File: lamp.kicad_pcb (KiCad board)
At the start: 2 copper layers, 83.8 x 40.6 mm, 18 parts, among them J1 Screw_Terminal_01x02, J2 Screw_Terminal_01x02, Q1 2N7002, U1 ESP-12E, U2 34.81-7048, U3 AMS1117-3.3

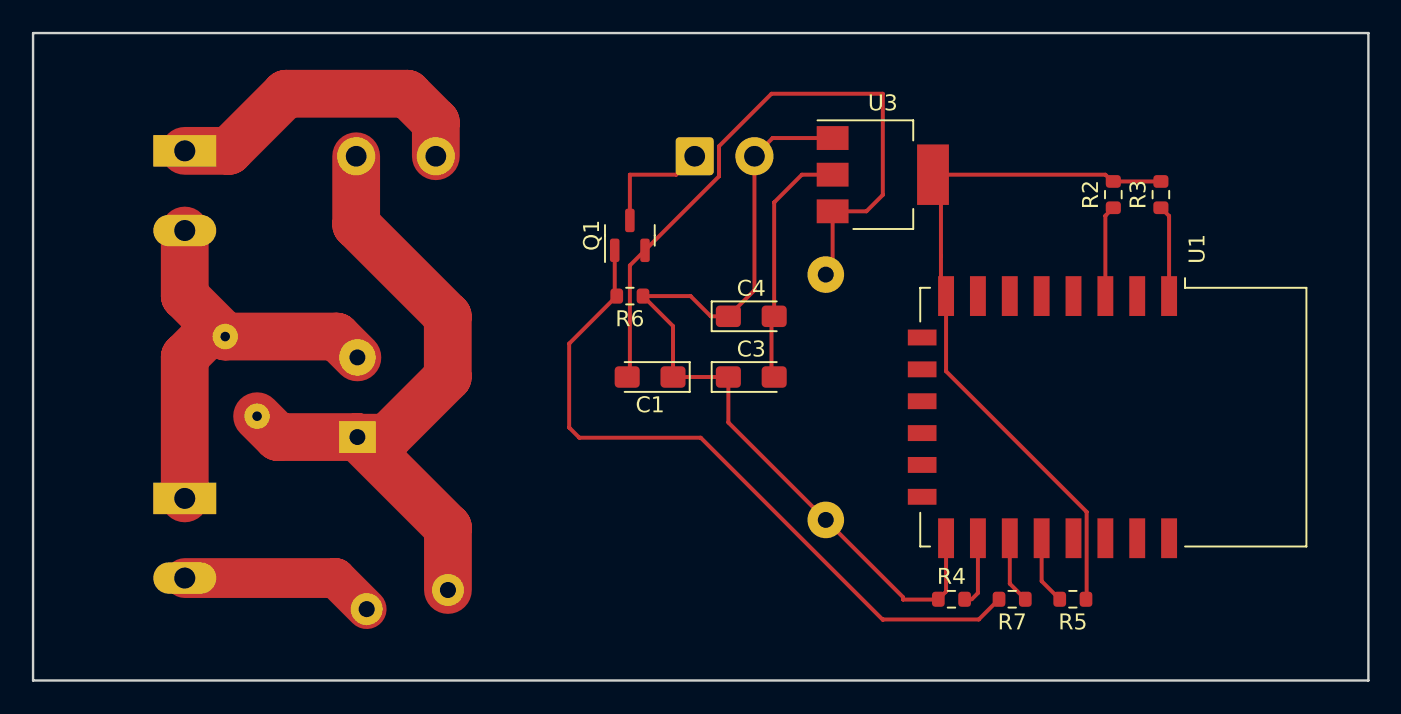
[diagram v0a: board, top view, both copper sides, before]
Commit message: some chnges
some changes
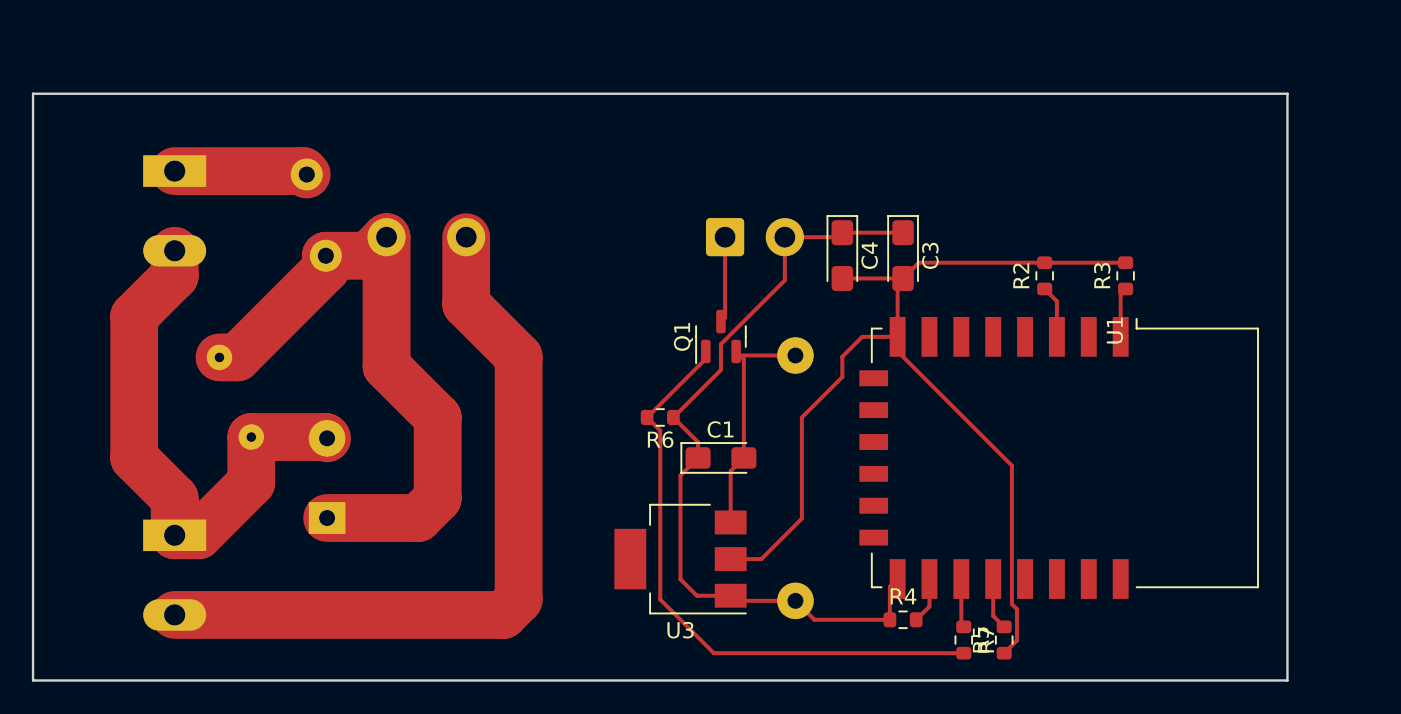
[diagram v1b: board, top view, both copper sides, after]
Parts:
- moved F1 27.5 mm to (130.2, 100.3), turned to -90 degrees
- moved U3 27.3 mm to (153.7, 124.5), turned to 180 degrees
- moved J1 24.1 mm to (121.9, 123.0)
- moved J2 20.6 mm to (121.9, 100.1)
- moved C3 12.2 mm to (167.6, 105.4), turned to -90 degrees
- moved Q1 8.54 mm to (156.2, 110.5)
- moved R6 7.86 mm to (152.4, 115.6)
- moved C4 6.87 mm to (163.8, 105.4), turned to -90 degrees
- moved C1 6.75 mm to (156.2, 118.1), turned to 0 degrees
- moved R2 6.68 mm to (176.5, 106.7)
- moved RV1 6.52 mm to (126.7, 116.8), turned to 90 degrees
- moved R3 5.56 mm to (181.6, 106.7)
- moved U2 5.43 mm to (156.5, 104.3)
- moved PS1 5.42 mm to (131.5, 121.9)
- moved R5 5.01 mm to (174.0, 129.5), turned to 90 degrees
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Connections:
- F1 pad 1: Net-(J2-Pad2) -> Net-(F1-Pad1)
- J1 pad 2: Net-(J2-Pad1) -> Net-(U2-Pad11)
- J2 pad 1: Net-(J2-Pad1) -> Net-(F1-Pad1)
- J2 pad 2: Net-(J2-Pad2) -> Net-(J1-Pad1)
- PS1 pad 2: Net-(J2-Pad1) -> Net-(J1-Pad1)
- RV1 pad 1: Net-(J2-Pad1) -> Net-(J1-Pad1)
- U2 pad 11: Net-(J1-Pad1) -> Net-(U2-Pad11)
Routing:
- net Net-(U2-Pad11): track 0.00 -> 46.1 mm
- net Net-(J2-Pad1): track 28.5 -> 0.00 mm
- net Net-(C1-Pad2): track 42.6 -> 15.1 mm
- net Net-(J1-Pad1): track 20.1 -> 33.8 mm
- net Net-(J2-Pad2): track 12.2 -> 0.00 mm
- net Net-(F1-Pad1): track 0.00 -> 8.38 mm
- net Net-(Q1-Pad1): track 44.9 -> 37.9 mm
- net Net-(C3-Pad2): track 59.3 -> 66.0 mm
- net GND: track 56.4 -> 50.0 mm
- net Net-(F1-Pad2): track 42.3 -> 39.3 mm
- net Net-(R3-Pad1): track 5.76 -> 3.13 mm
- net Net-(R2-Pad1): track 5.75 -> 3.32 mm
- net Net-(Q1-Pad3): track 7.42 -> 5.41 mm
- net Net-(R4-Pad2): track 4.44 -> 2.91 mm
- net Net-(R7-Pad1): track 4.23 -> 3.07 mm
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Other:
- board size 83.8 x 40.6 mm -> 78.7 x 36.8 mm
